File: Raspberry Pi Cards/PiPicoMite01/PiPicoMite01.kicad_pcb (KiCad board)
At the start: 2 copper layers, 69.8 x 120.7 mm, 45 parts, among them J1 Conn, SD Card, J2 USB-B, J3 HEADER, 1x20, J4 Conn_02x02_Odd_Even, J5 HEADER, 1x20, J6 Conn_02x10_Odd_Even, J7 AudioJack3, J8 PS2_DIN6, J9 Conn_02x03_Odd_Even, P1 CONN, DB15HD, BLUE (VGA), U1 RPi-PICO, U2 MCP23017_SP, U3 TXS0104

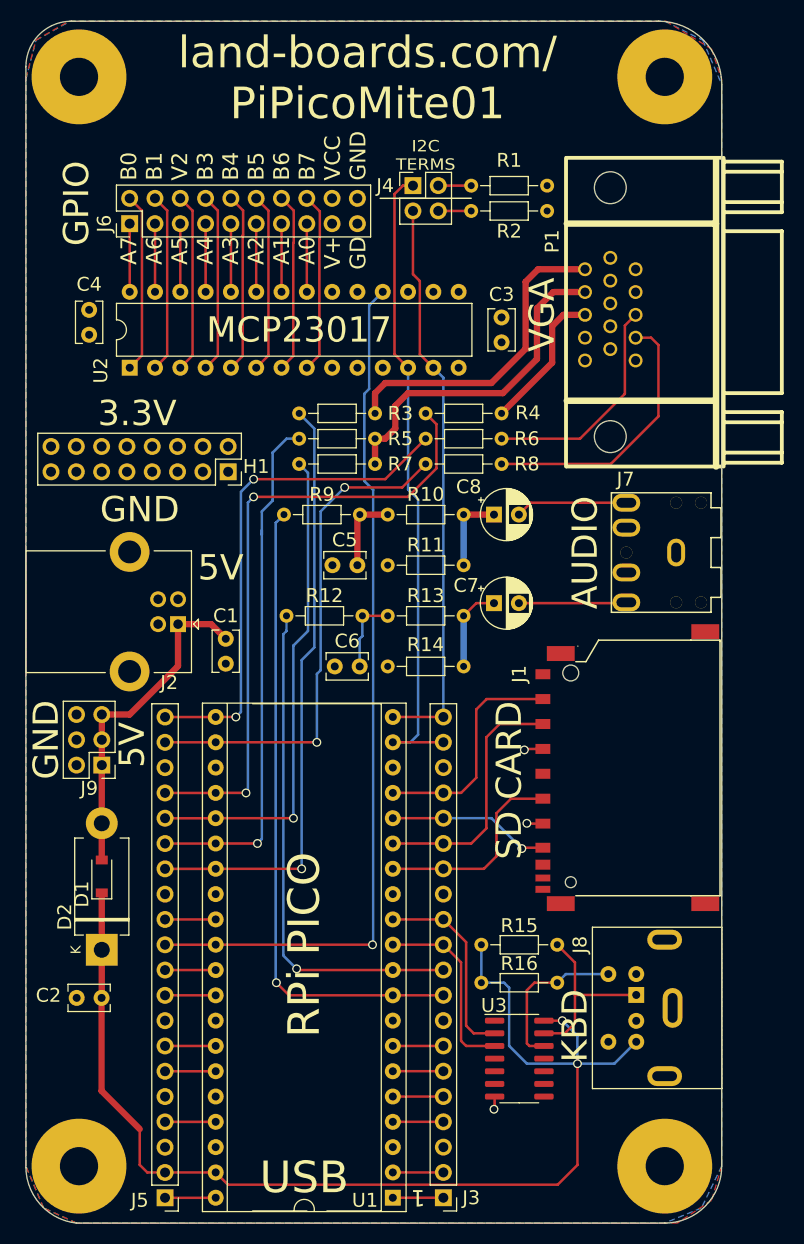
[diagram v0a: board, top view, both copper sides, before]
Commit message: Card updates
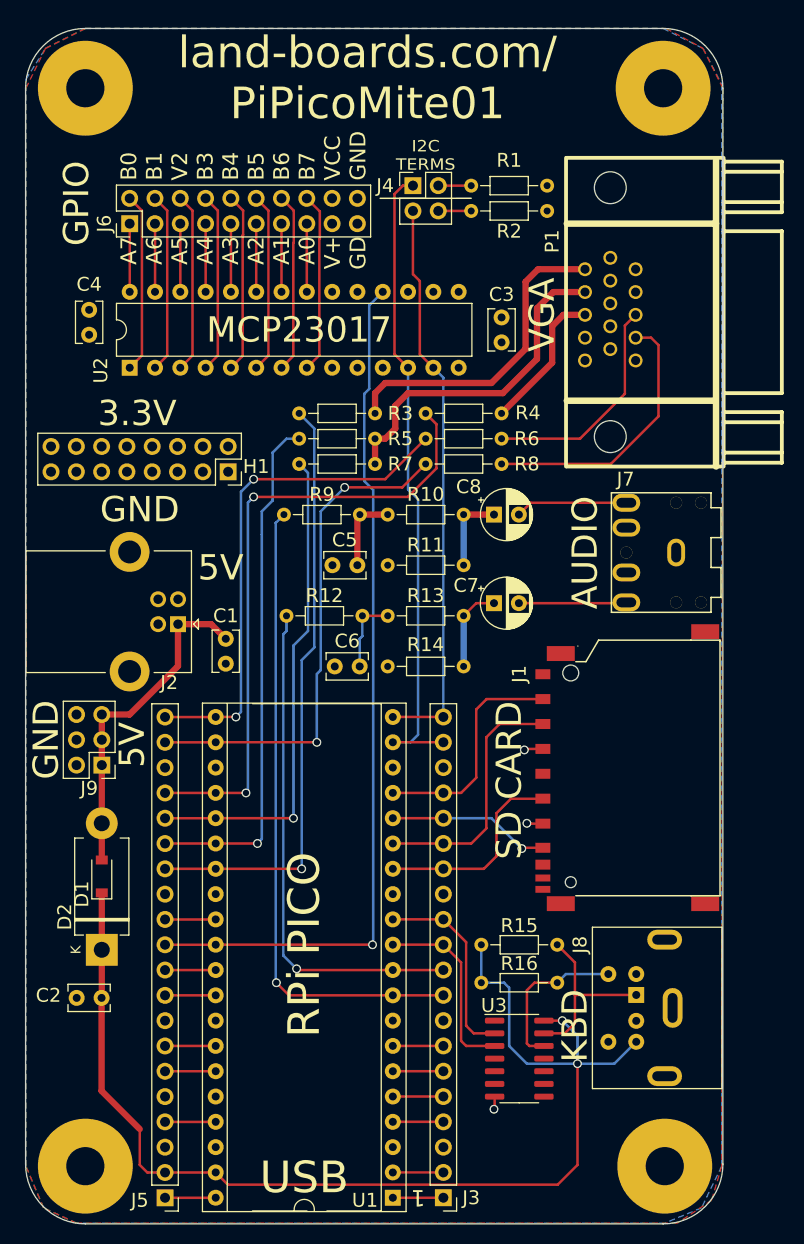
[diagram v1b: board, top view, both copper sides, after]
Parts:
- moved MTG1 1.31 mm to (119.0, 8.00)
- moved MTG3 1.15 mm to (177.0, 8.00)
- moved MTG4 0.64 mm to (119.0, 116.2)
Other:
- board size 69.8 x 120.7 mm -> 70 x 120 mm
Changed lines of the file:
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@@
   (net 88 "/VSYS")
   (footprint "LandBoards_MountHoles:MTG-6-32" (layer "F.Cu")
-    (at 118.364 6.858)
+    (at 119 8)
     (property "Sheetfile" "PiPicoMite01.kicad_sch")
     (property "Sheetname" "")
@@
   )
   (footprint "LandBoards_MountHoles:MTG-6-32" (layer "F.Cu")
-    (at 118.364 116.205)
+    (at 119 116.205)
     (property "Sheetfile" "PiPicoMite01.kicad_sch")
     (property "Sheetname" "")
@@
   )
   (footprint "LandBoards_MountHoles:MTG-6-32" (layer "F.Cu")
-    (at 177.165 6.858)
+    (at 177 8)
     (property "Sheetfile" "PiPicoMite01.kicad_sch")
     (property "Sheetname" "")
@@
   (gr_line (start 148.59 19.05) (end 157.734 19.05) (layer "B.SilkS") (width 0.15))
   (gr_line (start 148.59 19.05) (end 157.734 19.045) (layer "F.SilkS") (width 0.15))
-  (gr_line (start 113.03 116.332) (end 113.03 5.842) (layer "Edge.Cuts") (width 0.1))
-  (gr_arc (start 176.53 1.27) (mid 181.020128 3.129872) (end 182.88 7.62) (layer "Edge.Cuts") (width 0.1))
-  (gr_line (start 117.602 1.27) (end 176.53 1.27) (layer "Edge.Cuts") (width 0.1))
-  (gr_arc (start 118.11 121.92) (mid 114.512141 120.08769) (end 113.03 116.332) (layer "Edge.Cuts") (width 0.1))
-  (gr_arc (start 182.88 116.205) (mid 181.206115 120.246115) (end 177.165 121.92) (layer "Edge.Cuts") (width 0.1))
-  (gr_line (start 177.165 121.92) (end 118.11 121.92) (layer "Edge.Cuts") (width 0.1))
-  (gr_arc (start 113.03 5.842) (mid 114.369108 2.609108) (end 117.602 1.27) (layer "Edge.Cuts") (width 0.1))
-  (gr_line (start 182.88 116.205) (end 182.88 7.62) (layer "Edge.Cuts") (width 0.1))
+  (gr_line (start 177 2) (end 119 2) (layer "Edge.Cuts") (width 0.1))
+  (gr_arc (start 177 2) (mid 181.242641 3.757359) (end 183 8) (layer "Edge.Cuts") (width 0.1))
+  (gr_arc (start 119 122) (mid 114.757359 120.242641) (end 113 116) (layer "Edge.Cuts") (width 0.1))
+  (gr_line (start 113 8) (end 113 116) (layer "Edge.Cuts") (width 0.1))
+  (gr_arc (start 183 116) (mid 181.242641 120.242641) (end 177 122) (layer "Edge.Cuts") (width 0.1))
+  (gr_line (start 183 116) (end 183 8) (layer "Edge.Cuts") (width 0.1))
+  (gr_line (start 119 122) (end 177 122) (layer "Edge.Cuts") (width 0.1))
+  (gr_arc (start 113 8) (mid 114.757359 3.757359) (end 119 2) (layer "Edge.Cuts") (width 0.1))
   (gr_text "GND" (at 115.062 73.406 90) (layer "B.SilkS")
     (effects (font (size 2.54 2.54) (thickness 0.635)) (justify mirror))
@@
     (effects (font (size 2.54 2.54) (thickness 0.635)) (justify mirror))
   )
-  (gr_text "AUDIO" (at 175.514 47.498) (layer "B.SilkS")
+  (gr_text "AUDIO" (at 174 47.498) (layer "B.SilkS")
     (effects (font (size 1.4732 1.5875) (thickness 0.3048)) (justify right mirror))
   )
@@
   )
   (dimension (type aligned) (layer "Dwgs.User")
-    (pts (xy 118.872 121.92) (xy 118.364 1.27))
-    (height -8.89206)
-    (gr_text "4.7500 in" (at 110.876009 61.627598 -89.75875604) (layer "Dwgs.User")
-      (effects (font (size 1 1) (thickness 0.15)))
+    (pts (xy 113 8) (xy 183 8))
+    (height -13)
+    (gr_text "70.0000 mm" (at 148 -6.75) (layer "Dwgs.User")
+      (effects (font (size 1.5 1.5) (thickness 0.25)))
     )
     (format (units 3) (units_format 1) (precision 4))
@@
   )
   (dimension (type aligned) (layer "Dwgs.User")
-    (pts (xy 113.03 6.858) (xy 182.88 7.112))
-    (height -8.88717)
-    (gr_text "2.7500 in" (at 147.991499 -3.052103 359.7916526) (layer "Dwgs.User")
-      (effects (font (size 1 1) (thickness 0.15)))
+    (pts (xy 119 8) (xy 119 116))
+    (height 9)
+    (gr_text "108.0000 mm" (at 108.25 62 90) (layer "Dwgs.User")
+      (effects (font (size 1.5 1.5) (thickness 0.25)))
+    )
+    (format (units 3) (units_format 1) (precision 4))
+    (style (thickness 0.1) (arrow_length 1.27) (text_position_mode 0) (extension_height 0.58642) (extension_offset 0.5) keep_text_aligned)
+  )
+  (dimension (type aligned) (layer "Dwgs.User")
+    (pts (xy 119 2) (xy 119 122))
+    (height 15)
+    (gr_text "120.0000 mm" (at 102.25 62 90) (layer "Dwgs.User")
+      (effects (font (size 1.5 1.5) (thickness 0.25)))
+    )
+    (format (units 3) (units_format 1) (precision 4))
+    (style (thickness 0.1) (arrow_length 1.27) (text_position_mode 0) (extension_height 0.58642) (extension_offset 0.5) keep_text_aligned)
+  )
+  (dimension (type aligned) (layer "Dwgs.User")
+    (pts (xy 119 8) (xy 177 8))
+    (height -9)
+    (gr_text "58.0000 mm" (at 148 -2.75) (layer "Dwgs.User")
+      (effects (font (size 1.5 1.5) (thickness 0.25)))
     )
     (format (units 3) (units_format 1) (precision 4))
@@
   (segment (start 136.715011 50.482989) (end 137.795 49.403) (width 0.254) (layer "B.Cu") (net 40))
   (segment (start 137.795 49.403) (end 137.795 44.577) (width 0.254) (layer "B.Cu") (net 40))
-  (segment (start 136.715011 52.768989) (end 136.715011 52.387011) (width 0.254) (layer "B.Cu") (net 40))
   (segment (start 136.715011 83.365989) (end 136.715011 52.768989) (width 0.254) (layer "B.Cu") (net 40))
   (segment (start 139.192 43.18) (end 140.462 43.18) (width 0.254) (layer "B.Cu") (net 40))
@@
     (polygon
       (pts
-        (xy 181.864 4.064)
-        (xy 182.88 7.112)
+        (xy 181 4)
+        (xy 183 8)
         (xy 182.88 116.205)
         (xy 181.864 119.634)
@@
         (xy 114.808 120.396)
         (xy 113.03 116.205)
-        (xy 113.03 6.985)
-        (xy 114.046 3.175)
-        (xy 117.348 1.27)
-        (xy 177.292 1.27)
+        (xy 113.03 8)
+        (xy 115 4)
+        (xy 119 2)
+        (xy 177.292 2)
       )
     )
@@
     (polygon
       (pts
-        (xy 180.975 3.175)
+        (xy 181 4)
         (xy 182.88 7.62)
         (xy 182.88 116.205)
@@
         (xy 113.03 116.205)
         (xy 113.03 7.112)
-        (xy 114.046 3.175)
-        (xy 117.475 1.27)
-        (xy 177.165 1.27)
+        (xy 115 4)
+        (xy 119 2)
+        (xy 177 2)
       )
     )
